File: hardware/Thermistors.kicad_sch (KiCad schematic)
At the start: 10 parts, among them J1 Conn_01x08

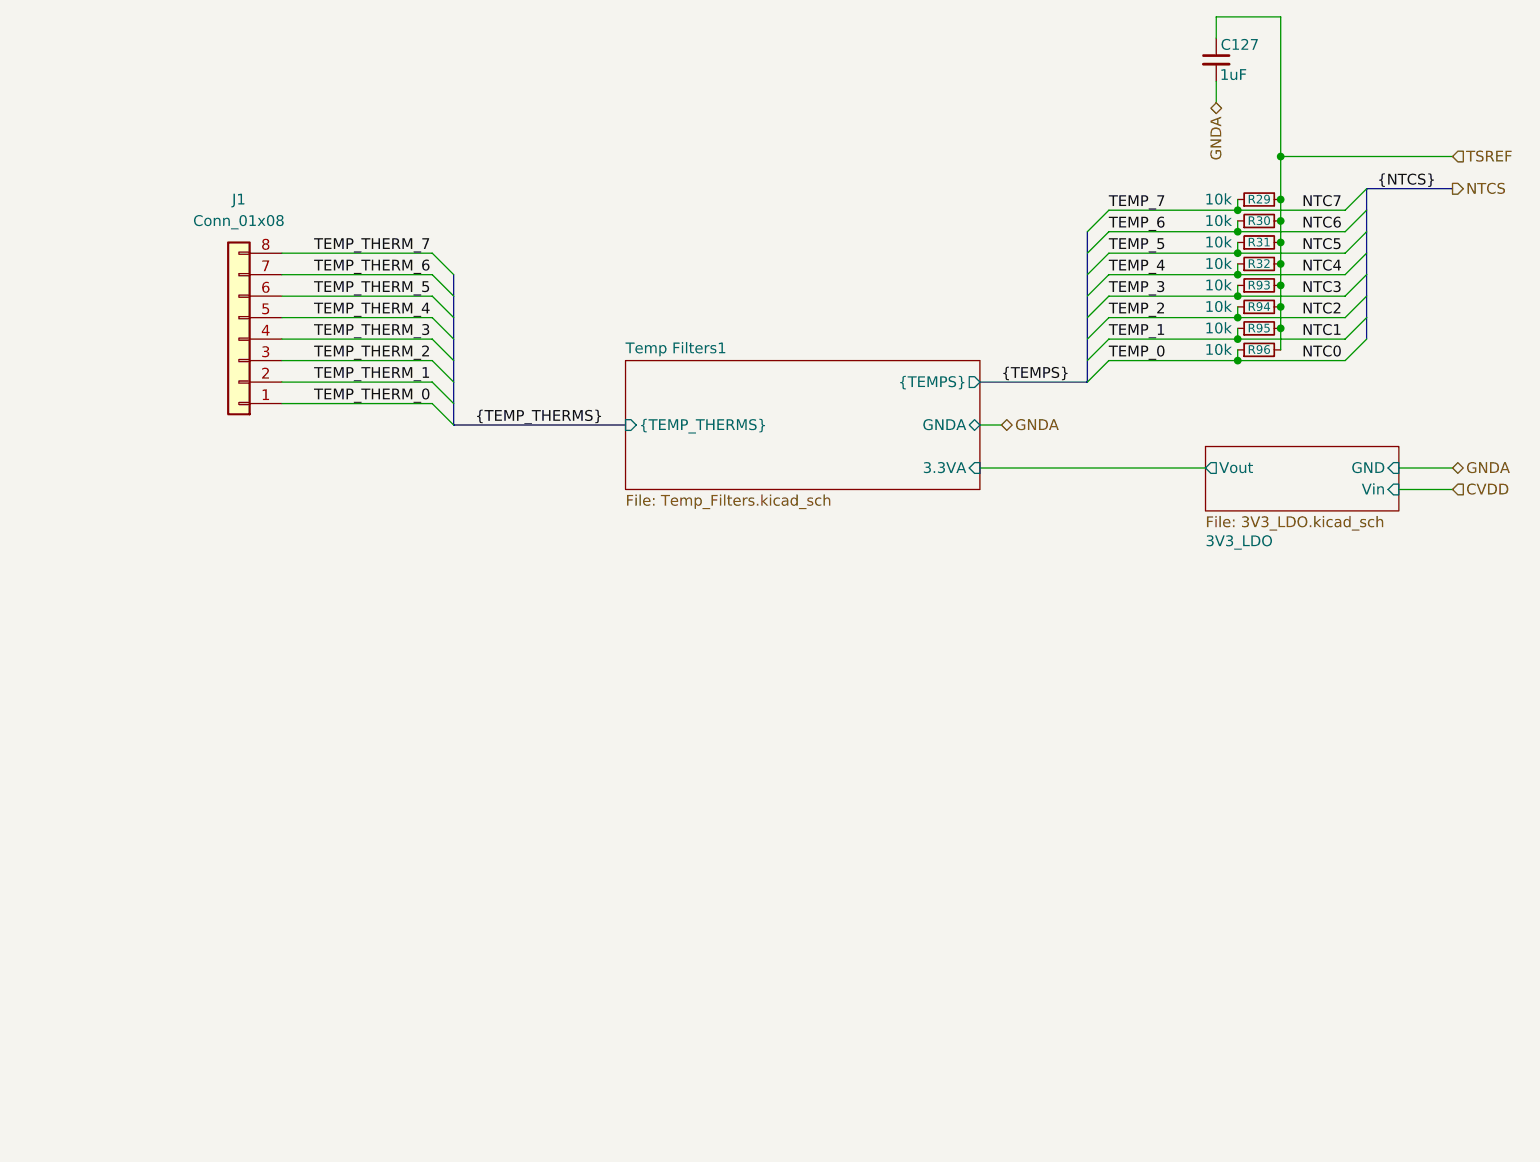
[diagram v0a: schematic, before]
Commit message: updated sheets and 1st review changes
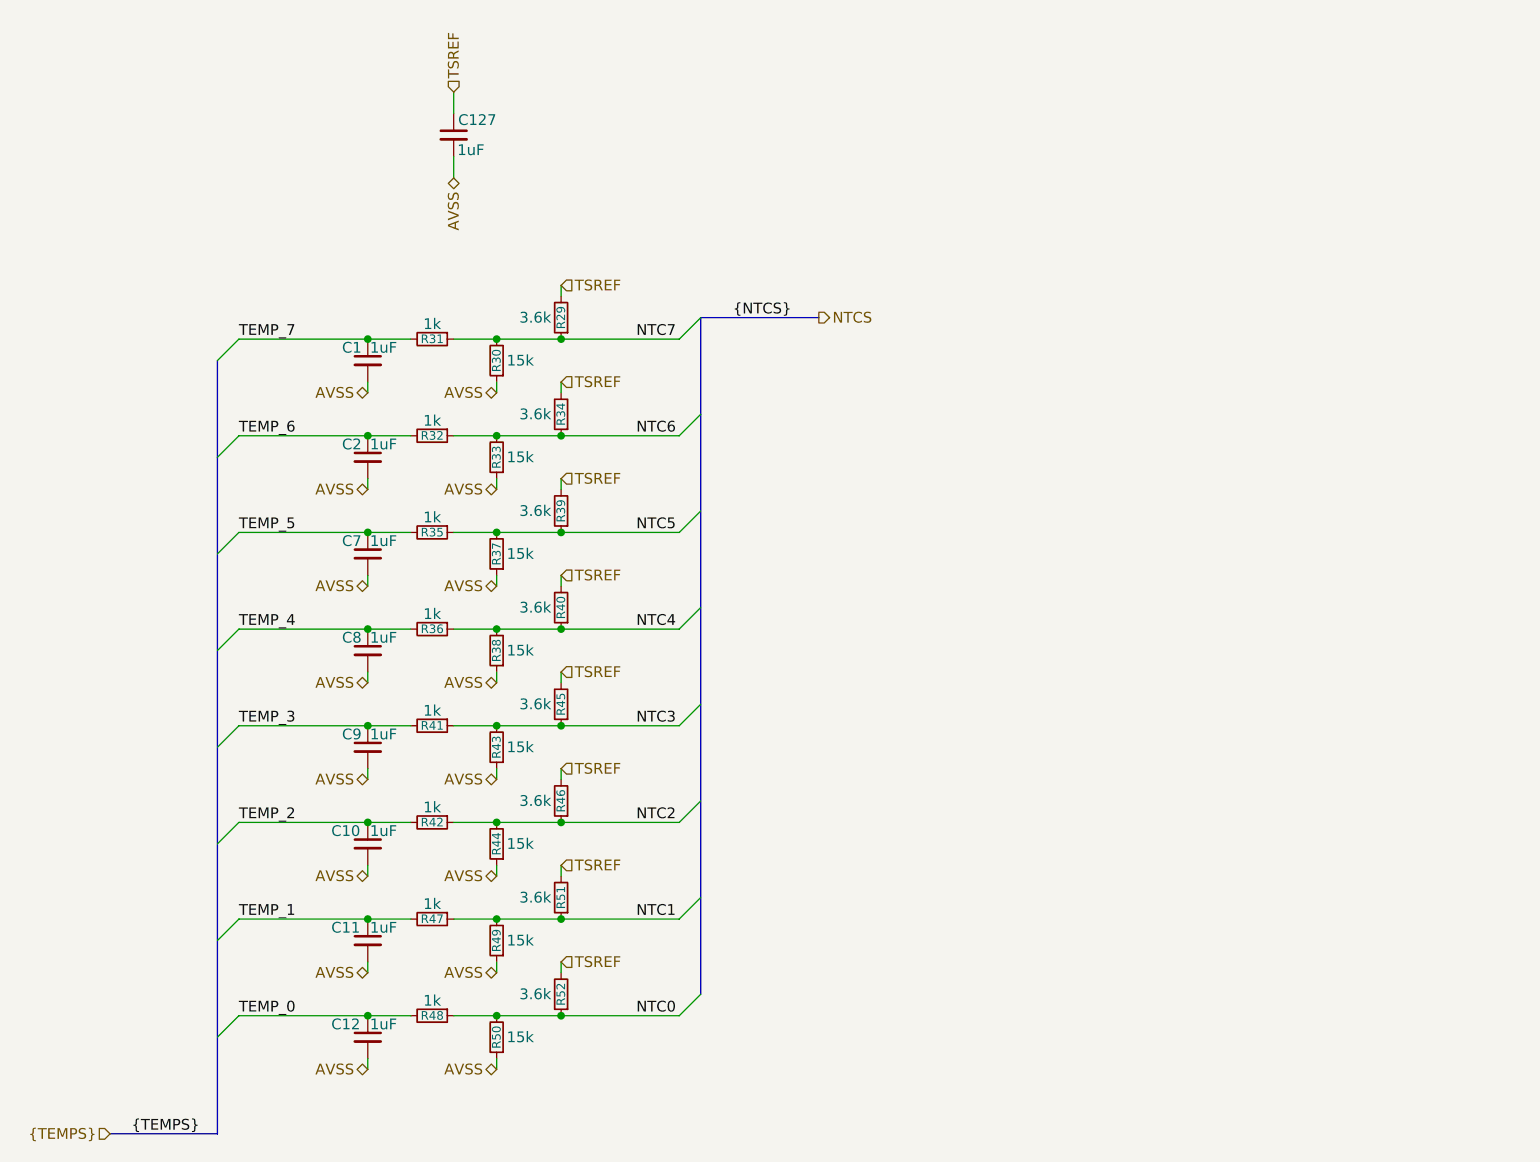
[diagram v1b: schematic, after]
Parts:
- removed J1: Conn_01x08, symbol Connector_Generic:Conn_01x08
- removed R93, R94, R95, R96: 10k, symbol Device:R_Small
- added C1, C10, C11, C12, C2, C7, C8, C9: 1uF, symbol Device:C_Small
- added R33, R37, R38, R43, R44, R49, R50: 15k, symbol Device:R_Small
- added R34, R39, R40, R45, R46, R51, R52: 3.6k, symbol Device:R_Small
- added R35, R36, R41, R42, R47, R48: 1k, symbol Device:R_Small
- R29: value 10k -> 3.6k
- R30: value 10k -> 15k
- R31, R32: value 10k -> 1k
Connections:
- net NTC0: now also R48.1, R50.2, R52.1
- net NTC1: now also R47.1, R49.2, R51.1
- net NTC2: now also R42.1, R44.2, R46.1
- net NTC3: now also R41.1, R43.2, R45.1
- net NTC4: now also R36.1, R38.2, R40.1; no longer R32.1
- net NTC5: now also R35.1, R37.2, R39.1; no longer R31.1
- net NTC6: now also R32.1, R33.2, R34.1; no longer R30.1
- net NTC7: now also R30.2, R31.1
- net TSREF: now also R34.2, R39.2, R40.2, R45.2, R46.2, R51.2, R52.2; no longer R30.2, R31.2, R32.2
- net GNDA renamed AVSS
- net AVSS: now also R30.1, C1.2, C10.2, C11.2, C12.2, C2.2, C7.2, C8.2, C9.2, R33.1, R37.1, R38.1, R43.1, R44.1, R49.1, R50.1
- new net TEMP_0: C12.1, R48.2
- new net TEMP_1: C11.1, R47.2
- new net TEMP_2: C10.1, R42.2
- new net TEMP_3: C9.1, R41.2
- new net TEMP_4: C8.1, R36.2
- new net TEMP_5: C7.1, R35.2
- new net TEMP_6: C2.1, R32.2
- new net TEMP_7: C1.1, R31.2
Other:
- removed sheet 3V3_LDO
- removed sheet Temp Filters1
- moved on the sheet: C127
